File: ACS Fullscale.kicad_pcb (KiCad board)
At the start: 2 copper layers, 151.1 x 151.1 mm, 35 parts, among them J1 Pulse-20, J2 Conn_01x02, U1 SN65HVD230, U10 BNO086, U11 R-78E5.0-1.0, U2 MS5611-01BA, U4 Teensy4.1, U5 TPS62202DBV, U6 BHI360, U7 TXS0108EPW, U8 BMP581, U9 BME280, Y1 32.768k

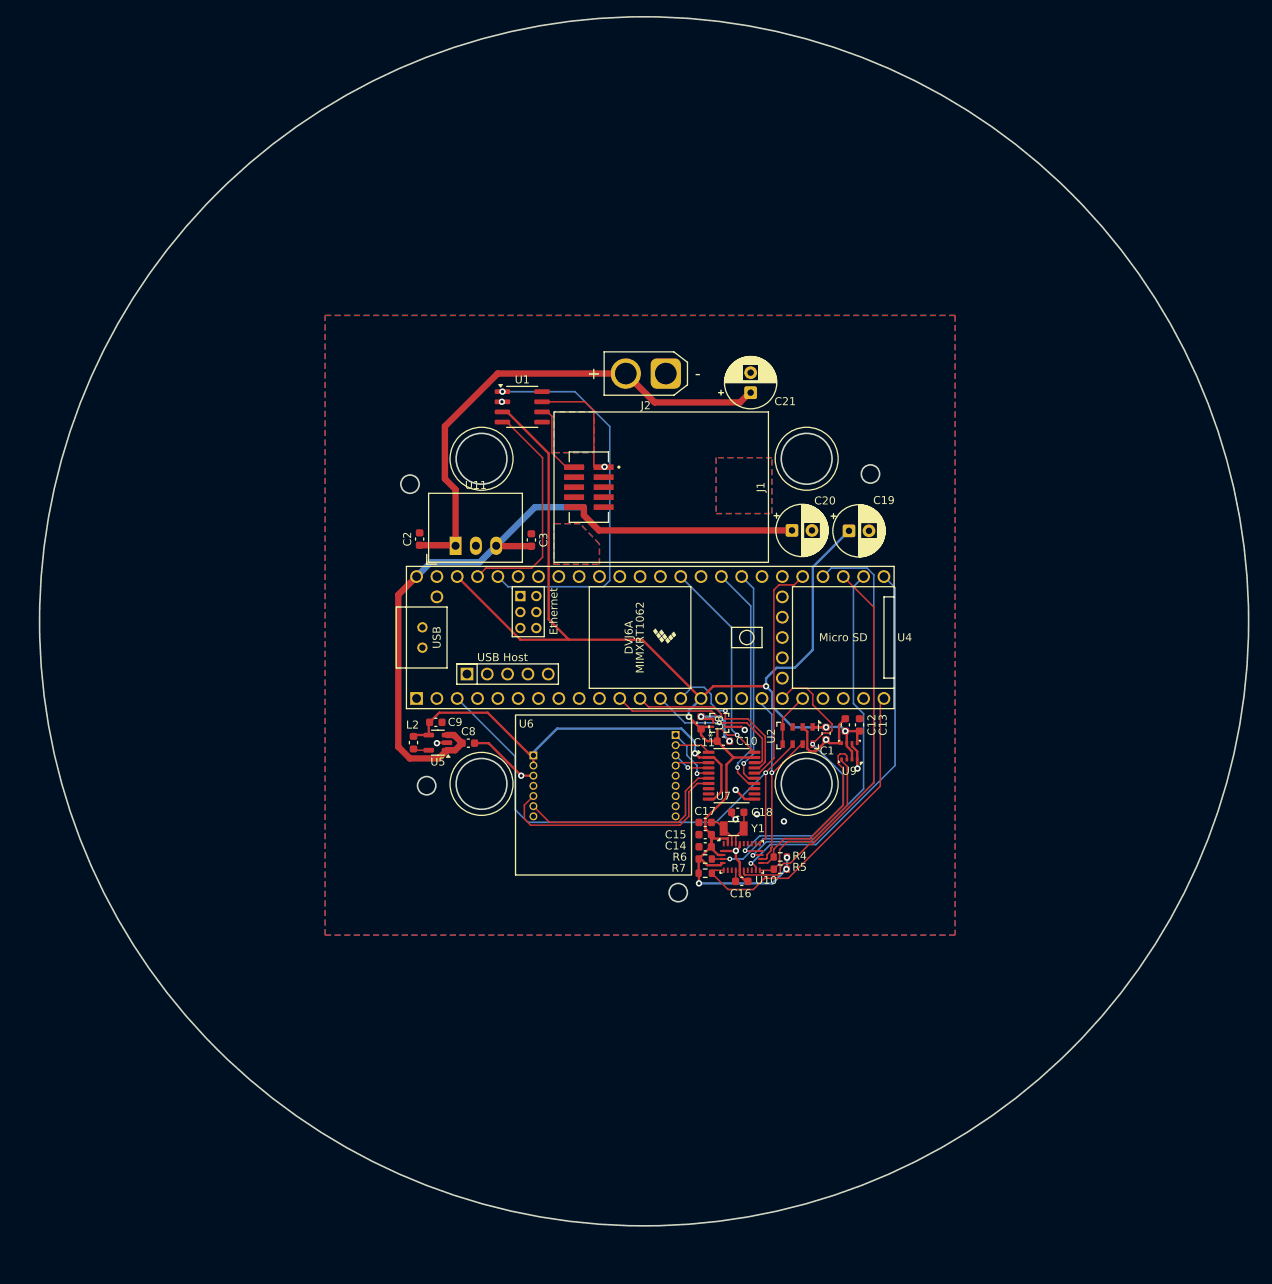
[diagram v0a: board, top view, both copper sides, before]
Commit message: A lot of stuff
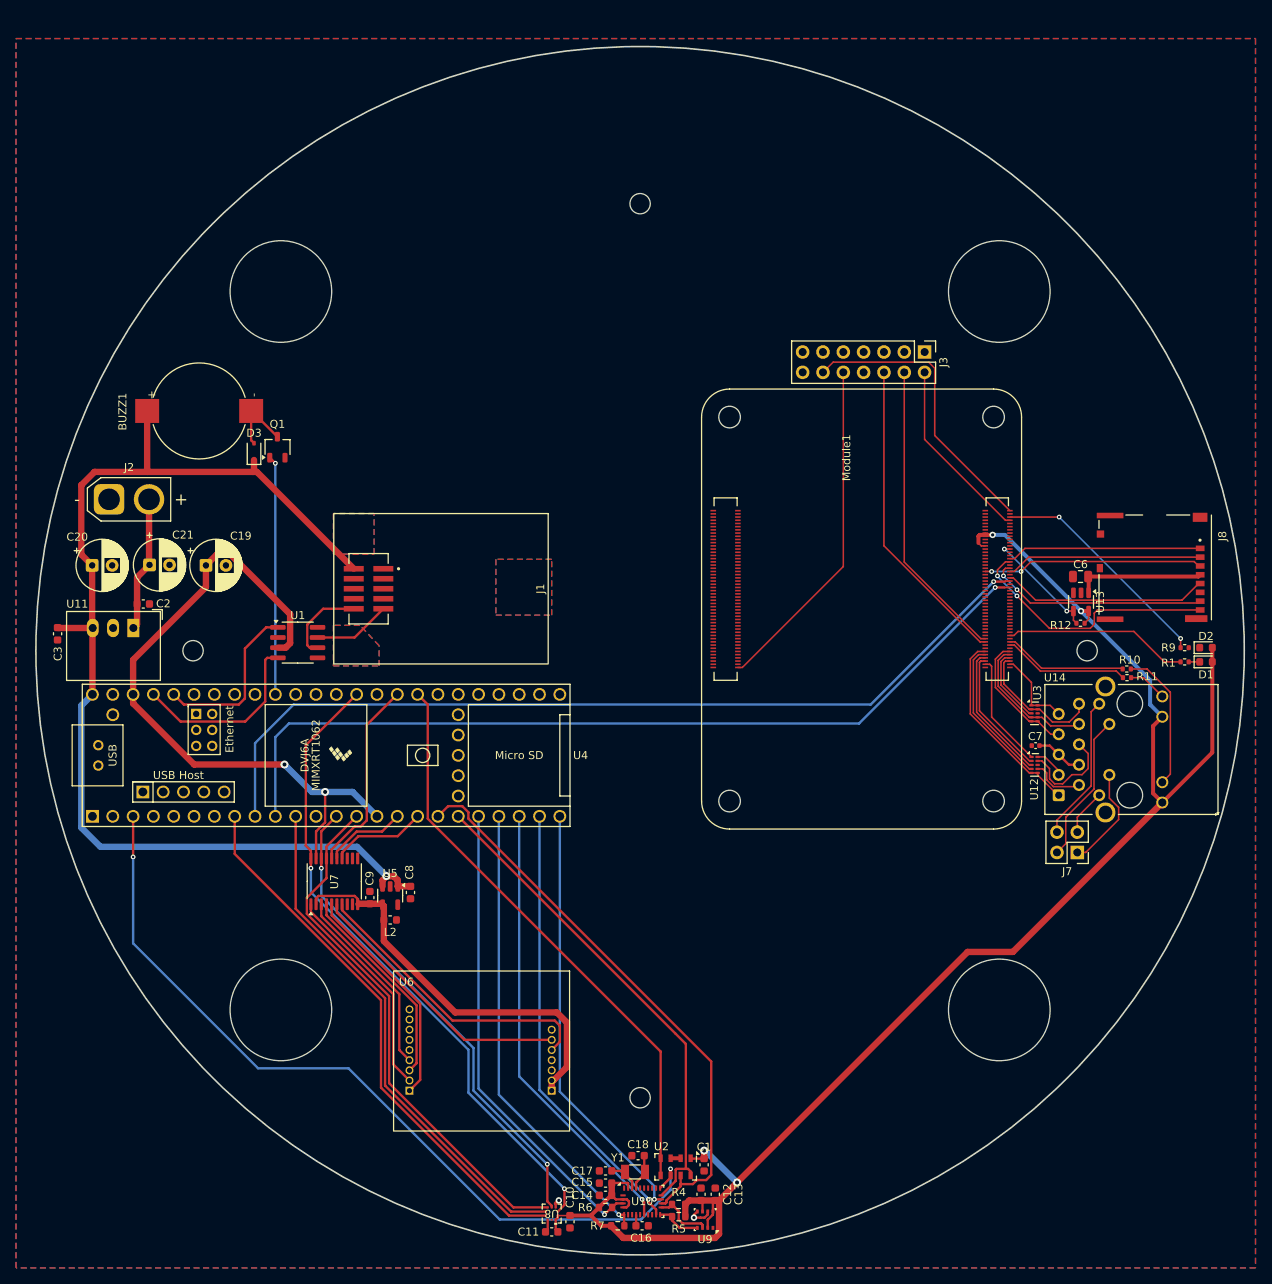
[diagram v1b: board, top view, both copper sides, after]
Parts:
- added BUZZ1: CD-1206-SMT, ACS_Footprint_Library:CUI_CD-1206-SMT, F.Cu at (97.3, 69.1)
- added C6: 10u, Capacitor_SMD:C_0805_2012Metric, F.Cu at (207.5, 89.8)
- added C7: 100n, Capacitor_SMD:C_0402_1005Metric, F.Cu at (201.8, 110.9)
- added D1: LED Green, LED_SMD:LED_0603_1608Metric, F.Cu at (223.1, 100.5)
- added D2: LED Red, LED_SMD:LED_0603_1608Metric, F.Cu at (223.1, 98.7)
- added D3: D, Diode_SMD:D_SOD-323, F.Cu at (104.1, 74.2)
- added J3: Conn_02x07_Odd_Even, Connector_PinHeader_2.54mm:PinHeader_2x07_P2.54mm_Vertical, F.Cu at (188.0, 61.7)
- added J7: THD-02-R, Connector_PinHeader_2.54mm:PinHeader_2x02_P2.54mm_Vertical, F.Cu at (207.0, 124.3)
- added J8: Micro_SD_Card_Det, CM5IO:SDCARD_MOLEX_503398-1892, F.Cu at (216.8, 88.6)
- added Module1: ComputeModule5-CM5, CM5IO:Raspberry-Pi-5-Compute-Module, F.Cu at (196.6, 69.9)
- added Q1: Q_NPN_BEC, Package_TO_SOT_SMD:TSOT-23, F.Cu at (107.1, 73.6)
- added R1: 1k, Resistor_SMD:R_0402_1005Metric, F.Cu at (220.5, 100.5)
- added R10: 470R, Resistor_SMD:R_0402_1005Metric, F.Cu at (213.2, 101.3)
- added R11: 470R, Resistor_SMD:R_0402_1005Metric, F.Cu at (213.3, 102.4)
- added R12: 10K 1%, Resistor_SMD:R_0402_1005Metric, F.Cu at (207.5, 95.6)
- added R9: 1k, Resistor_SMD:R_0402_1005Metric, F.Cu at (220.5, 98.7)
- added U12: TPD4EUSB30, Package_SON:USON-10_2.5x1.0mm_P0.5mm, F.Cu at (201.7, 113.3)
- added U13: RT9742GGJ5, Package_TO_SOT_SMD:SOT-23-5, F.Cu at (207.5, 93.0)
- added U14: MagJack-A70-112-331N126, CM5IO:TRJG0926HENL, F.Cu at (213.6, 111.4)
- added U3: TPD4EUSB30, Package_SON:USON-10_2.5x1.0mm_P0.5mm, F.Cu at (201.7, 106.9)
- moved C20 87.6 mm to (83.9, 88.4)
- moved C19 80.5 mm to (98.1, 88.4)
- moved C21 78.2 mm to (91.1, 88.3), turned to 0 degrees
- moved J2 71.3 mm to (86.0, 80.1), turned to 0 degrees
- moved C11 66.3 mm to (141.4, 171.7), turned to 180 degrees
- moved U8 64.8 mm to (141.4, 169.4), turned to 180 degrees
- moved C10 63.1 mm to (143.6, 170.4), turned to -90 degrees
- moved C12 61.4 mm to (160.0, 167.0)
- moved C13 61.4 mm to (161.8, 167.0)
- moved U9 61.3 mm to (160.5, 170.2)
- moved C3 60.4 mm to (79.6, 96.9), turned to -90 degrees
- moved C1 56.0 mm to (160.4, 163.3)
- moved U2 56.0 mm to (156.8, 163.6)
- moved U7 51.4 mm to (114.2, 127.9), turned to 90 degrees
- moved R7 45.4 mm to (149.6, 170.9)
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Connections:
- U4 pad 10: unconnected-(U4-8_TX2_IN1-Pad10) -> /TX2
- U4 pad 11: /INT0 -> /CS0
- U4 pad 12: /CS0 -> unconnected-(U4-10_CS_MQSR-Pad12)
- U4 pad 16: unconnected-(U4-24_A10_TX6_SCL2-Pad16) -> /INT2
- U4 pad 17: unconnected-(U4-25_A11_RX6_SDA2-Pad17) -> /RST2
- U4 pad 20: /CS1 -> /BT3
- U4 pad 21: unconnected-(U4-29_TX7-Pad21) -> /WAKE3
- U4 pad 22: unconnected-(U4-30_CRX3-Pad22) -> /RST3
- U4 pad 23: unconnected-(U4-31_CTX3-Pad23) -> /INT3
- U4 pad 24: /WAKE3 -> /CS3
- U4 pad 25: /INT3 -> unconnected-(U4-33_MCLK2-Pad25)
- U4 pad 26: /BT3 -> unconnected-(U4-34_RX8-Pad26)
- U4 pad 27: /RST3 -> unconnected-(U4-35_TX8-Pad27)
- U4 pad 28: /CS3 -> unconnected-(U4-36_CS-Pad28)
- U4 pad 29: /CS2 -> unconnected-(U4-37_CS-Pad29)
- U4 pad 32: /INT2 -> /CS1
- U4 pad 33: /RST2 -> /CS2
- U4 pad 39: unconnected-(U4-17_A3_TX4_SDA1-Pad39) -> /Buzz
- U4 pad 8: unconnected-(U4-6_OUT1D-Pad8) -> /INT0
- U4 pad 9: unconnected-(U4-7_RX2_OUT1A-Pad9) -> /RX2
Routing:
- net /RX2: track 0.00 -> 111.9 mm, vias 0 -> 1
- net +3V3: track 182.6 -> 293.8 mm, vias 7 -> 6
- net /TX2: track 0.00 -> 109.5 mm, vias 0 -> 1
- net /CS1: track 6.74 -> 72.7 mm
- net /INT0: track 13.1 -> 68.7 mm
- net /CS0: track 11.3 -> 64.9 mm
- net /SCK0: track 28.1 -> 81.0 mm, vias 1 -> 2
- net +5V: track 91.0 -> 143.4 mm, vias 0 -> 1
- net /MISO0: track 19.8 -> 66.4 mm, vias 1 -> 0
- net +BATT: track 63.0 -> 16.9 mm
- net /MOSI1: track 26.9 -> 71.7 mm, vias 1 -> 0
- net /MOSI0: track 18.7 -> 61.6 mm, vias 1 -> 2
- net /CM5_GPIO ( Ethernet, GPIO, SDCARD)/USBOTG: track 0.00 -> 42.7 mm
- net /CM5_GPIO ( Ethernet, GPIO, SDCARD)/SYNC_OUT: track 0.00 -> 39.3 mm
- net /MISO1: track 65.6 -> 104.5 mm, vias 1 -> 2
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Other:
- board size 151.1 x 151.1 mm -> 151 x 151 mm
